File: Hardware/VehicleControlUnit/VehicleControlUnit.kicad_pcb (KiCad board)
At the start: 4 copper layers, 100 x 80 mm, 220 parts, among them IC1 LM74502DDFR, IC2 TCAN3413DR, IC3 EMC2305-1-AP-TR, IC4 ISO7741DWR, IC5 ISO7741DWR, IC6 ISO7741DWR, IC7 ISO1042QDWRQ1, J1 CAN_DEBUG_NANO_01x04, J10 SWD_Header, J11 SWD, J12 Micro_SD_Card_Det2, J13 Debug_Conn, J14 USB_C_Receptacle_USB2.0_16P, J2 WaveSculptor Debug, J3 CAN_NANO_01x03, J4 Thermistor, J5 CAN_NANO_01x03, J6 Fan_Conn1, J7 MotorConn_1, J8 Motor_Conn2, J9 Fan_Conn2, Q1 PSMN012-100YS, Q2 PSMN012-100YS, Q3 IRLML2030TRPBF, Q4 DMP3099L-7, Q5 IRLML2030TRPBF, Q6 IRLML2030TRPBF, Q7 IRLML2030TRPBF, Q8 IRLML2030TRPBF, SW1 SW_SPDT, U1 LMR51635XDDCR, U2 TPS2117DRLR, U3 MCP1826S, U4 STM32G473VETx, U5 MCP4922T-E/ST, Y1 Crystal

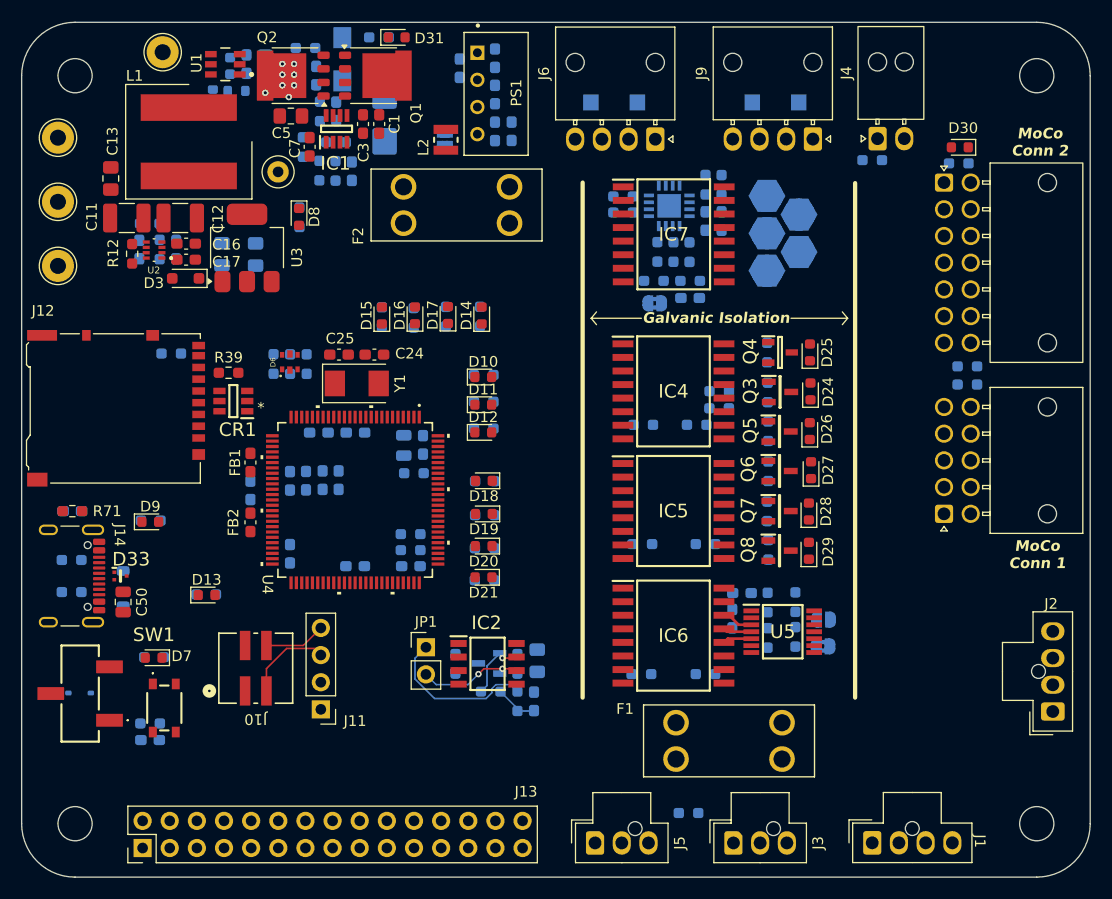
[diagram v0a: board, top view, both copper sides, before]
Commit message: migtve finally lcokeefd in = ggs
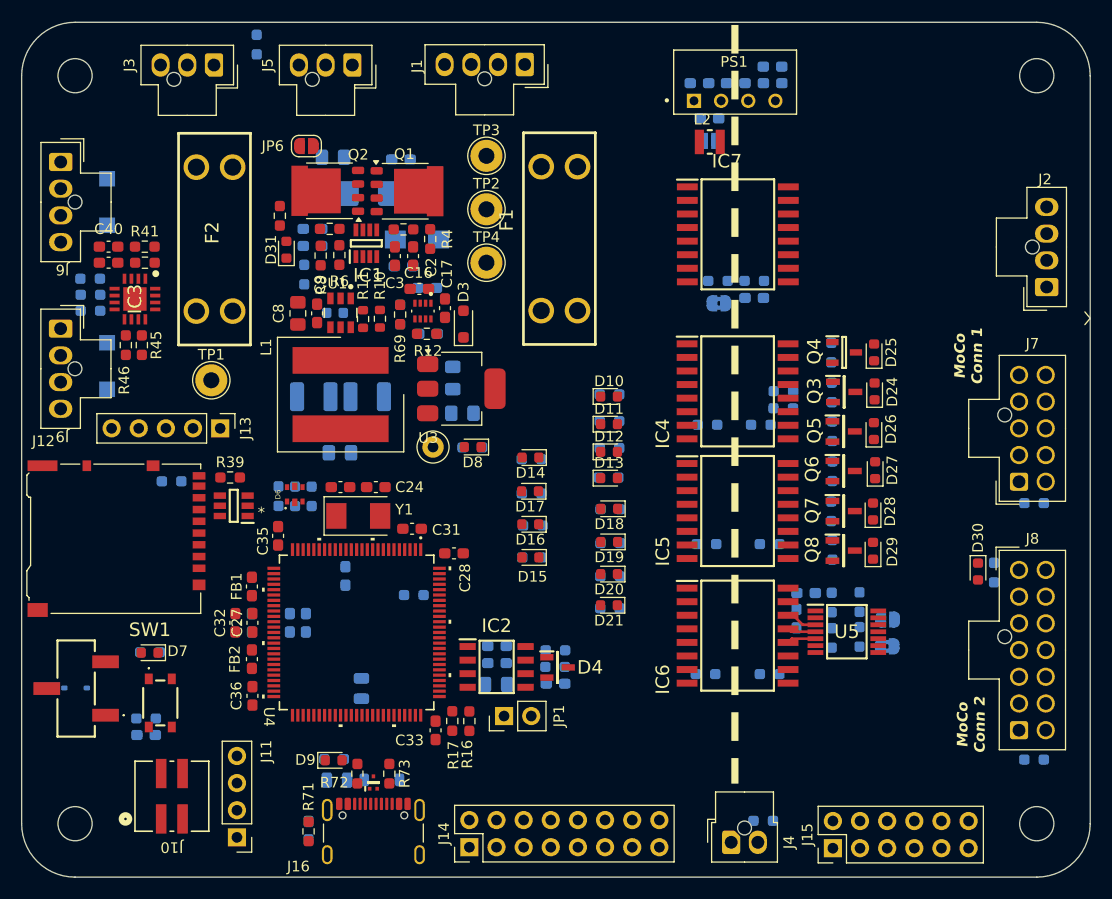
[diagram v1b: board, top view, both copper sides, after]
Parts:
- removed TP5, TP6, TP7, TP8, TP9: TestPoint, diddle_shah:TestPoint_HEX_3mmID
- added J14: Debug_Conn1, Connector_PinHeader_2.54mm:PinHeader_2x08_P2.54mm_Vertical, F.Cu at (131.9, 127.2)
- added J15: Debug_Conn2, Connector_PinHeader_2.54mm:PinHeader_2x06_P2.54mm_Vertical, F.Cu at (165.9, 127.3)
- added JP6: SolderJumper_2_Open, Jumper:SolderJumper-2_P1.3mm_Open_RoundedPad1.0x1.5mm, F.Cu at (116.7, 61.6)
- C1, C11, C12, C13, C5, C50, C7: moved to B.Cu
- C2, C27, C28, C31, C32, C33, C35, C36, C39, C40, C8, C9, D4, IC3, R10, R11, R16, R17, R4, R40, R41, R45, R46, R5, R6, R69, R7, R72, R73, R8, R9: moved to F.Cu
- F1, F2: footprint FuseHolder:FUSE_3568 -> LHRS_Power:Fuse-3557-2
- J13: value Debug_Conn -> Fan_Debug_Conn; footprint Connector_PinHeader_2.54mm:PinHeader_2x15_P2.54mm_Vertical -> Connector_PinHeader_2.54mm:PinHeader_1x05_P2.54mm_Vertical
- J4: footprint Connector_Molex:Molex_Nano-Fit_105313-xx02_1x02_P2.50mm_Horizontal -> LHRS_Connectors:Molex_Nano-Fit_105309-xx02_1x02_P2.50mm_Vertical
- J6, J9: footprint LHRS_Connectors:Molex_Nano-Fit_105313-xx04_1x04_P2.50mm_Horizontal -> LHRS_Connectors:Molex_Nano-Fit_105309-xx04_1x04_P2.50mm_Vertical
- J7: footprint LHRS_Connectors:Molex_Nano-Fit_105314-xx10_2x05_P2.50mm_Horizontal -> LHRS_Connectors:Molex_Nano-Fit_105310-xx10_2x05_P2.50mm_Vertical
- J8: footprint cutom_2x7_nanofit:nanofit_2x7_diff_pinouts -> cutom_2x7_nanofit:custom_2x07_vertical_nanofit
- PS1: value ROE-3.305S -> ROE-3.505S
- moved J3 93.5 mm to (103.0, 54.0), turned to 90 degrees
- moved J1 83.3 mm to (132.7, 54.2), turned to 90 degrees
- moved R1 82.5 mm to (112.0, 52.1), turned to 90 degrees
- moved J5 79.8 mm to (116.0, 54.0), turned to 90 degrees
- moved D23 67.2 mm to (98.0, 82.2), turned to -90 degrees
- moved J4 66.8 mm to (158.9, 126.7), turned to -90 degrees
- moved J9 66.4 mm to (93.9, 83.1), turned to 180 degrees
- moved R23 62.7 mm to (159.4, 124.7), turned to 0 degrees
- moved C40 57.4 mm to (98.1, 71.0), turned to 180 degrees
- moved R42 56.1 mm to (96.4, 74.0), turned to 0 degrees
- moved C39 56.0 mm to (98.1, 72.5), turned to 180 degrees
- moved R43 54.7 mm to (96.4, 75.5), turned to 180 degrees
- moved R41 54.3 mm to (101.5, 71.0), turned to 0 degrees
- moved R44 53.3 mm to (96.4, 77.0), turned to 180 degrees
- moved R40 53.0 mm to (101.5, 72.5), turned to 0 degrees
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- renumbered J14 to J16
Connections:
- net /Motor Comms/+3.3V_in renamed /Motor Comms/+5V_in
- net /Power Regulation/12VBuck/V_in renamed /Power Regulation/Vout_pp
- C17 pad 1: /Power Regulation/LDO/Vin -> +5V
- D3 pad 2: /Power Regulation/LDO/Vin -> +5V
- J13 pad 1: +3.3V -> /MCU + Peripherals/ALERT
- J13 pad 2: GND -> /FAN1_PWM
- J13 pad 3: /BrakeADC -> /FAN1_TACH
- J13 pad 4: /Accel_ADC -> /MCU + Peripherals/SDA
- J13 pad 5: /MCU + Peripherals/LDAC -> /MCU + Peripherals/SCL
- J7 pad 1: /Brake_Vref -> Net-(J7-Pin_1)
- J7 pad 10: Net-(J7-Pin_10) -> Net-(J7-Pin_1)
- J7 pad 2: /Accel_Vref -> /Mtr_Pulse
- J7 pad 4: /Mtr_Pulse -> /Accel_Vref
- J7 pad 5: Net-(J7-Pin_5) -> /Brake_Vref
- J7 pad 6: Net-(J7-Pin_5) -> Net-(J7-Pin_6)
- J7 pad 7: GND_ISO -> Net-(J7-Pin_6)
- J7 pad 9: Net-(J7-Pin_10) -> GND_ISO
- J8 pad 1: /Moco_LED+ -> Net-(J8-Pin_1)
- J8 pad 10: /map_bit1_sig -> /FR_MODE_IN
- J8 pad 12: /FR_MODE_IN -> /map_bit1_sig
- J8 pad 13: /PWR_MODE_OUT -> /map_bit3_sig
- J8 pad 14: /Moco_LED- -> Net-(J8-Pin_1)
- J8 pad 2: /PWR_MODE_IN -> /map_bit2_sig
- J8 pad 3: /FR_MODE_OUT -> /map_bit0_sig
- J8 pad 5: /map_bit0_sig -> /FR_MODE_OUT
- J8 pad 6: /map_bit2_sig -> /PWR_MODE_IN
- J8 pad 7: Net-(J8-Pin_7) -> /Moco_LED+
- J8 pad 8: Net-(J8-Pin_7) -> /Moco_LED-
- J8 pad 9: /map_bit3_sig -> /PWR_MODE_OUT
- JP5 pad 1: +3.3V -> +5V
- L2 pad 1: +3.3V -> +5V
- R2 pad 1: Net-(J7-Pin_5) -> Net-(J7-Pin_1)
- R3 pad 1: Net-(J8-Pin_7) -> Net-(J8-Pin_1)
- U2 pad 2: /Power Regulation/LDO/Vin -> +5V
- U2 pad 7: /Power Regulation/LDO/Vin -> +5V
- U4 pad 55: /MCU + Peripherals/100PinMCU/PD8 -> /MCU + Peripherals/ESTOP_Fault
- U4 pad 56: /MCU + Peripherals/100PinMCU/PD9 -> /MCU + Peripherals/SWOC
- U4 pad 88: /MCU + Peripherals/100PinMCU/PD6 -> /MCU + Peripherals/Mtr_Fault
- U4 pad 89: /MCU + Peripherals/100PinMCU/PD7 -> /MCU + Peripherals/BPS_Fault
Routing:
- net Net-(JP1-A): track 14.8 -> 0.00 mm
- net /CarCAN_L: track 10.1 -> 0.00 mm, vias 2 -> 0
- net Net-(J10-Pin_3): track 8.21 -> 0.00 mm
- net /CarCAN_H: track 6.22 -> 0.00 mm, vias 1 -> 0
- net Net-(J10-Pin_4): track 5.77 -> 0.00 mm
- net Net-(C23-Pad2): track 4.04 -> 0.00 mm
- net /Power Regulation/Vout_pp: vias 8 -> 0
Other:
- board text removed: "Galvanic Isolation"
